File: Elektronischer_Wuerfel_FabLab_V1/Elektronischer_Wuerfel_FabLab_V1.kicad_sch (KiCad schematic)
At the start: 20 parts, among them J1 Conn_01x02_Socket, J2 Conn_01x01_Socket, J3 Conn_01x06_Socket, U1 ATtiny85-20S

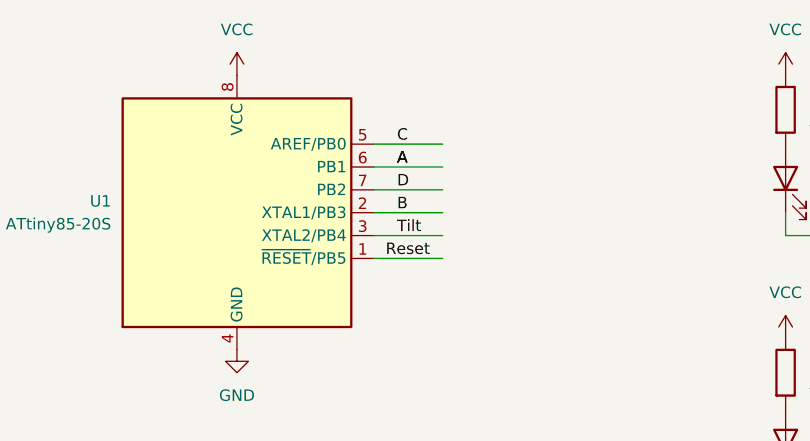
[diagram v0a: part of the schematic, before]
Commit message: some minor changes, repair of not connected A
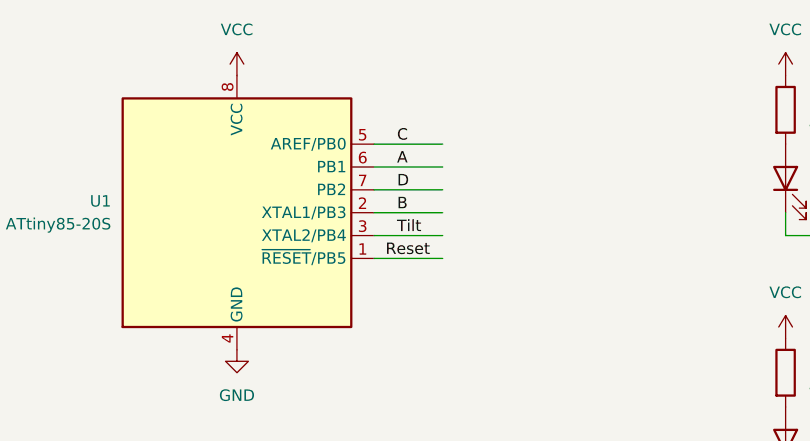
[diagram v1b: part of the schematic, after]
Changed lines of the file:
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@@
-		)
-	)
-	(label "A"
-		(at 144.78 60.96 0)
-		(fields_autoplaced yes)
-		(effects
-			(font
-				(size 1.27 1.27)
-			)
-			(justify left bottom)
 		)
 	)
